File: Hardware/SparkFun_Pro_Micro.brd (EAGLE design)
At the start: 17.8 x 33 mm, 33 parts, among them U2 MIC5219, U3 ATMEGA32U4, Y1 16MHz

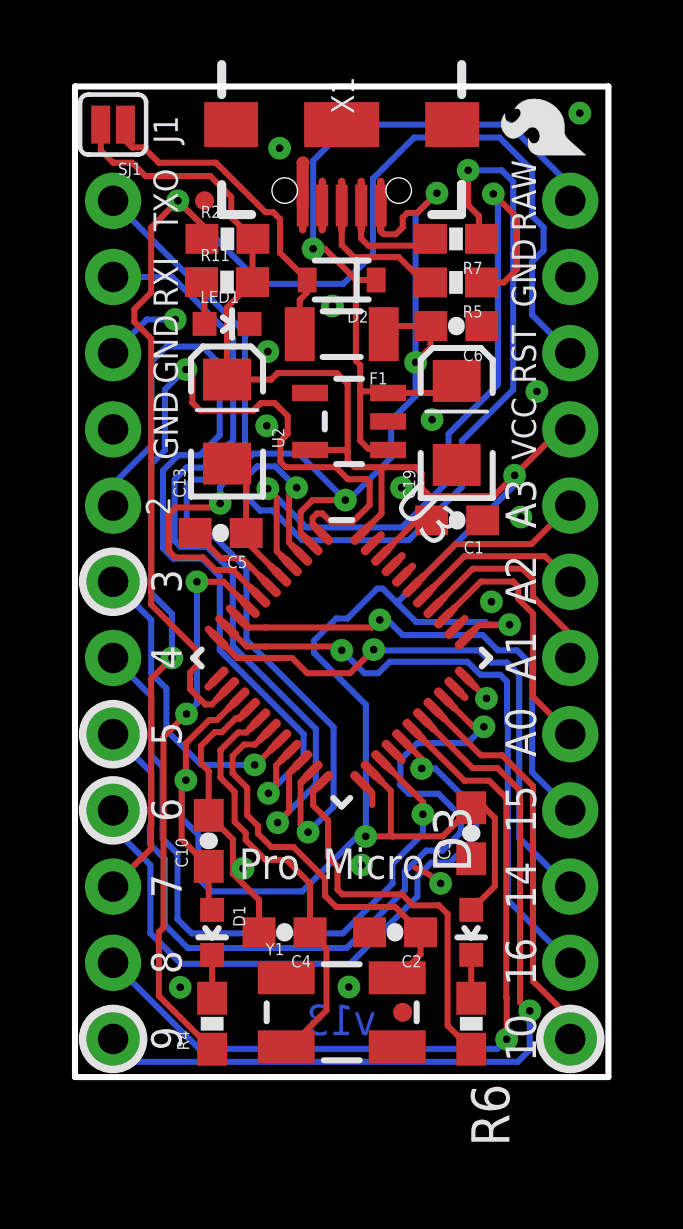
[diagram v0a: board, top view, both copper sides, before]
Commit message: Proto finished. Add ignore.
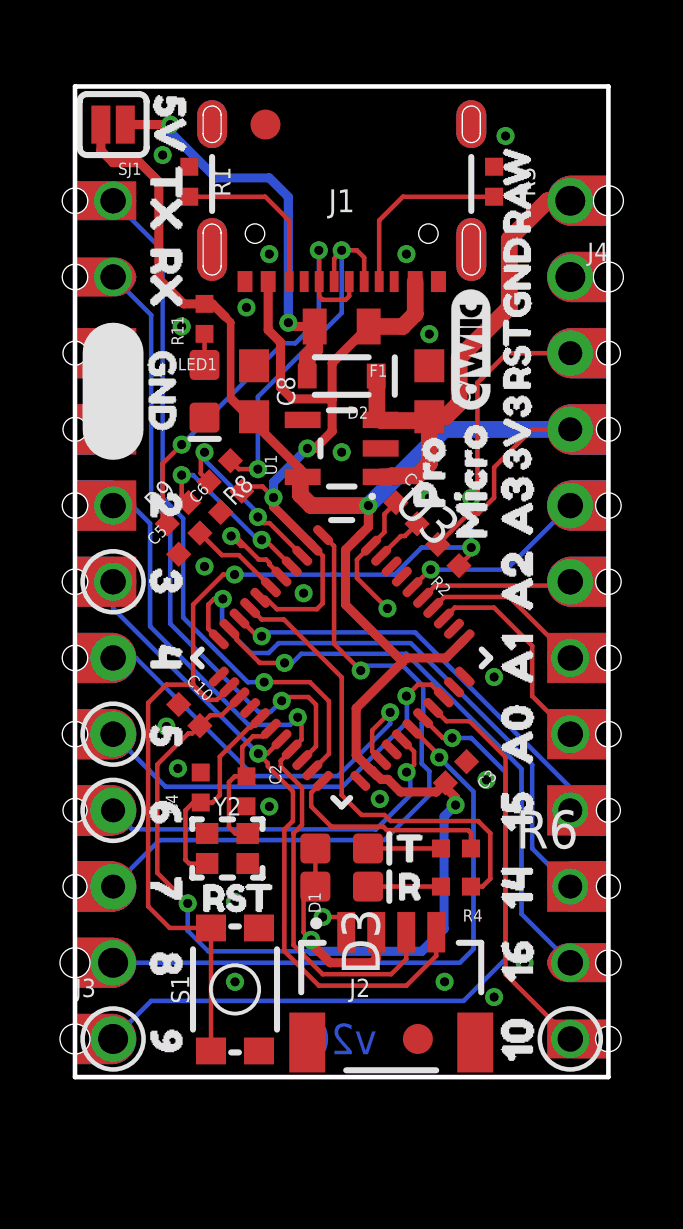
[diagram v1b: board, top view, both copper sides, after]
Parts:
- removed C13, C19: 10uF, SparkFun:EIA3216
- removed JP6, JP7: (no value), SparkFun:1X12
- removed R5, R7: 22, SparkFun:0603-RES
- removed U2: MIC5219, SparkFun:SOT23-5
- removed X1: (no value), Testing:USB-AB-MICRO-SMD-V03-IN&OUT
- removed Y1: 16MHz, SparkFun:CRYSTAL-SMD-5X3
- added C7, C8: 10uF, SparkFun-Capacitors:0603
- added J1: (no value), USBC:USB-C-16P-4
- added J2: Qwiic, SparkFun-Connectors:JST04_1MM_RA
- added J3, J4: (no value), Castellated:1X12_CASTELLATED
- added LOGO1: SFE_LOGO_NAME_FLAME.1_INCH, SparkFun-Aesthetics:SFE_LOGO_NAME_FLAME_.1
- added LOGO2: QWIIC_LOGO_4MM, SparkFun-Aesthetics:QWIIC_4MM
- added LOGO3: QWIIC_LOGO_6MM, SparkFun-Aesthetics:QWIIC_6MM
- added R1, R3: 5.1k, SparkFun-Resistors:0402-TIGHT
- added R8, R9: 22, SparkFun-Resistors:0402-TIGHT
- added S1: Reset, SparkFun-Switches:TACTILE_SWITCH_SMD_4.6X2.8MM
- added U$10, U$51: (no value), buzzard_labels (15):812
- added U$12, U$46: (no value), buzzard_labels (17):RAW5
- added U$13, U$55: (no value), buzzard_labels (13):45
- added U$14: (no value), buzzard_labels (17):T8
- added U$15, U$33: (no value), buzzard_labels (18):3V39
- added U$16, U$50: (no value), buzzard_labels (15):911
- added U$17, U$37: (no value), buzzard_labels (15):A07
- added U$18, U$60: (no value), buzzard_labels (13):TX2
- added U$19, U$36: (no value), buzzard_labels (15):A18
- added U$2, U$38: (no value), buzzard_labels (15):156
- added U$20: (no value), SparkFun-Aesthetics:PRODUCTION_INSTRUCTIONS
- added U$21, U$49: (no value), buzzard_labels (14):104
- added U$22, U$32: (no value), buzzard_labels (17):GND4
- added U$23: (no value), buzzard_labels (14):MICRO1
- added U$24: (no value), buzzard_labels (14):PRO0
- added U$25: (no value), buzzard_labels (16):RST3
- added U$26, U$35: (no value), buzzard_labels (15):A29
- added U$27, U$34: (no value), buzzard_labels (15):A310
- added U$28, U$59: (no value), buzzard_labels (15):RX20
- added U$29, U$47: (no value), buzzard_labels (15):145
- added U$30: (no value), buzzard_labels (17):R9
- added U$31, U$41: (no value), buzzard_labels (17):RST3
- added U$4, U$48: (no value), buzzard_labels (15):164
- added U$40: (no value), buzzard_labels (18):C5
- added U$43: (no value), buzzard_labels (18):MICRO4
- added U$45: (no value), buzzard_labels (18):PRO3
- added U$5, U$57: (no value), buzzard_labels (15):218
- added U$52, U$9: (no value), buzzard_labels (15):713
- added U$53, U$8: (no value), buzzard_labels (15):614
- added U$54, U$7: (no value), buzzard_labels (15):515
- added U$56, U$6: (no value), buzzard_labels (15):317
- added U$58: (no value), buzzard_labels (16):GND4
- added U1: 3.3V, SparkFun-IC-Power:SOT23-5
- added Y2: 32MHz, SparkFun-Clocks:CRYSTAL-SMD-2.0X1.6MM
- C1, C2, C3, C4: device SparkFun:0603-CAP -> SparkFun-Capacitors:0402-TIGHT
- C10, C5, C6: value 1uF -> 1.0uF; device SparkFun:0603-CAP -> SparkFun-Capacitors:0402-TIGHT
- D1: device SparkFun:LED-0603 -> SparkFun-LED:LED-0603
- D2: value (none) -> 3A/10V/280mV; device SparkFun:SOD-323 -> SparkFun-DiscreteSemi:SOD-323
- D3: value Green -> GREEN; device SparkFun:LED-0603 -> SparkFun-LED:LED-0603
- F1: value 500mA -> 6V 0.5A; device SparkFun:PTC-1206 -> SparkFun-Fuses:0805
- JP1, JP2: value FIDUCIALUFIDUCIAL -> FIDUCIAL1X2; device SparkFun:MICRO-FIDUCIAL -> SparkFun-Aesthetics:FIDUCIAL-1X2
- LED1: value Red -> RED; device SparkFun:LED-0603 -> SparkFun-LED:LED-0603
- R11: value 1K -> 1k; device SparkFun:0603-RES -> SparkFun-Resistors:0402-TIGHT
- R2: value 10K -> 10k; device SparkFun:0603-RES -> SparkFun-Resistors:0402-TIGHT
- R4, R6: value 330 -> 1k; device SparkFun:0603-RES -> SparkFun-Resistors:0402-TIGHT
- SJ1: device SparkFun:SJ_2S -> SparkFun-Jumpers:SMT-JUMPER_2_NO_SILK
- U$1: value LOGO-SFESK -> (none); device SparkFun:SFE-LOGO-FLAME -> buzzard_labels (15):5V21
- U$11: value LOGO-SFENEW -> (none); device SparkFun:SFE-NEW-WEBLOGO -> buzzard_labels (16):GND4
- U$3: value OSHW-LOGOS -> OSHW-LOGOMINI; device SparkFun:OSHW-LOGO-S -> SparkFun-Aesthetics:OSHW-LOGO-MINI
- U3: value ATMEGA32U4 -> ATmega32U4; device Testing:QFN-44-NOPAD_1:1-OUTFAKES -> SparkFun-IC-Microcontroller:QFN-44-NOPAD_1:1
- moved U$3 19.3 mm to (16.3, 31.5), turned to 0 degrees
- moved U$11 18.9 mm to (2.92, 25.1), flipped to the top, turned to 270 degrees
- moved U$1 14.1 mm to (3.17, 33.7), turned to 270 degrees
- moved R2 12.9 mm to (12.4, 17.4), turned to 135 degrees
- moved C6 9.52 mm to (5.21, 19.2), turned to 45 degrees
- moved R4 9.33 mm to (12.7, 6.35), turned to 180 degrees
- moved C2 6.83 mm to (5.71, 9.53), turned to 270 degrees
- moved R6 5.86 mm to (12.7, 7.62), turned to 180 degrees
- moved C4 5.58 mm to (4.19, 9.65), turned to 90 degrees
- moved D3 5.14 mm to (8.89, 7.62), turned to 0 degrees
- moved D1 4.58 mm to (8.89, 6.35), turned to 0 degrees
- moved C10 4.24 mm to (3.81, 12.1), turned to 315 degrees
- moved JP2 3.25 mm to (6.35, 31.8)
- moved D2 3.20 mm to (8.89, 23.4)
- moved LED1 2.37 mm to (4.32, 22.9)
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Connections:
- net D14 renamed RXLED
- net N$4 renamed UCAP
- removed net A4: U3.40
- removed net A5: U3.41
- removed net D11: U3.12
- removed net D12: U3.26
- removed net D13: U3.32
- removed net D2: JP7.8, U3.19
- removed net D3: JP7.7, U3.18
- removed net N$6: R7.2, X1.D-1
- removed net N$8: R5.2, X1.D+1
- removed net UVCC: C6.2, F1.1, U3.2, U3.7, X1.VBUS1
- new net D-_HV: J1.A7, J1.B7, R8.1
- new net D2/SDA: J2.3, J3.8, U3.19
- new net D3/SCL: J2.4, J3.7, U3.18
- new net DP_HV: J1.A6, J1.B6, R9.1
- new net N$10: J1.B5, R1.2
- new net N$9: J1.A5, R3.2
- new net USB_RAW: D2.A, F1.2, SJ1.1
- new net V_USB: C6.2, F1.1, J1.VBUS1, J1.VBUS2, U3.2, U3.7
- net A0: now also J4.8; no longer JP6.8
- net A1: now also J4.7; no longer JP6.7
- net A2: now also J4.6; no longer JP6.6
- net A3: now also J4.5; no longer JP6.5
- net D+: now also R9.2; no longer R5.1
- net D-: now also R8.2; no longer R7.1
- net D10: now also J4.12; no longer JP6.12
- net D4: now also J3.6; no longer JP7.6
- net D5: now also J3.5; no longer JP7.5
- net D6: now also J3.4; no longer JP7.4
- net D7: now also J3.3; no longer JP7.3
- net D8: now also J3.2; no longer JP7.2
- net D9: now also J3.1; no longer JP7.1
- net GND: now also C10.1, C7.1, C8.1, J1.GND, J1.GND2, J2.1, J3.9, J4.2, R1.1, R3.1, S1.1, S1.2, U1.2; no longer C10.2, C13.C, C19.C, JP6.2, JP7.10, JP7.9, U2.2, X1.GND1
- net MISO: now also J4.10; no longer JP6.10
- net MOSI: now also J4.11; no longer JP6.11
- net N$1: now also Y2.1; no longer Y1.1
- net N$2: now also Y2.3; no longer Y1.3
- net N$3: now also J3.10; no longer D2.2, F1.2, SJ1.1
- net RAW: now also C7.2, D2.C, J4.1, U1.1, U1.3; no longer C19.A, D2.1, JP6.1, U2.1, U2.3
- net RESET: now also J4.3, S1.3, S1.4; no longer JP6.3
- net RXI: now also J3.11; no longer JP7.11
- net SCK: now also J4.9; no longer JP6.9
- net TXO: now also J3.12; no longer JP7.12
- net VCC: now also C10.2, C8.2, J2.2, J4.4, U1.5; no longer C10.1, C13.A, JP6.4, U2.5
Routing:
- net UVCC: track 33.6 -> 0.00 mm, vias 4 -> 0
- net D2: track 27.8 -> 0.00 mm, vias 1 -> 0
- net D2/SDA: track 0.00 -> 24.9 mm, vias 0 -> 1
- net V_USB: track 0.00 -> 23.3 mm, vias 0 -> 2
- net D-: track 28.7 -> 6.07 mm
- net D3/SCL: track 0.00 -> 22.6 mm, vias 0 -> 1
- net D+: track 24.6 -> 5.94 mm
- net DP_HV: track 0.00 -> 14.7 mm, vias 0 -> 2
- net D5: track 27.6 -> 13.9 mm
- net USB_RAW: track 0.00 -> 13.5 mm, vias 0 -> 2
- net D-_HV: track 0.00 -> 12.3 mm, vias 0 -> 2
- net GND: track 20.0 -> 8.22 mm, vias 17 -> 25
- net N$3: track 11.1 -> 0.00 mm
- net D6: track 23.2 -> 12.8 mm
- net D3: track 9.86 -> 0.00 mm, vias 1 -> 0
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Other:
- board text added: "0.8mm PCB"
- board text added: "N. Seidle"
- board text added: "v20"
- board text removed: "10"
- board text removed: "14"
- board text removed: "15"
- board text removed: "16"
- board text removed: "2"
- board text removed: "3"
- board text removed: "3.3V"
- board text removed: "3.3V Reg / 8MHz"
- board text removed: "4"
- board text removed: "5"
- board text removed: "5V"
- board text removed: "5V Reg / 16MHz"
- board text removed: "6"
- board text removed: "7"
- board text removed: "8"
- board text removed: "9"
- board text removed: "A0"
- board text removed: "A1"
- board text removed: "A2"
- board text removed: "A3"
- board text removed: "GND"
- board text removed: "J1"
- board text removed: "Mark back accordingly"
- board text removed: "Micro"
- board text removed: "N. Seidle, revised by P. Lewis"
- board text removed: "Pro"
- board text removed: "RAW"
- board text removed: "RST"
- board text removed: "RXI"
- board text removed: "TXO"
- board text removed: "VCC"
- board text removed: "Valid combinations:"
- board text removed: "v13"
